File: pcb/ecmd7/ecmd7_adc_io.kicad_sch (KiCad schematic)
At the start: 72 parts, among them U10 FIN1002M5X, U11 FIN1002M5X, U12 FIN1002M5X, U13 ADM3490ExR, U2 MCP33151-05T-E/MN, U4 MCP33151-05T-E/MN, U5 MCP33151-05T-E/MN, U7 MCP33151-05T-E/MN

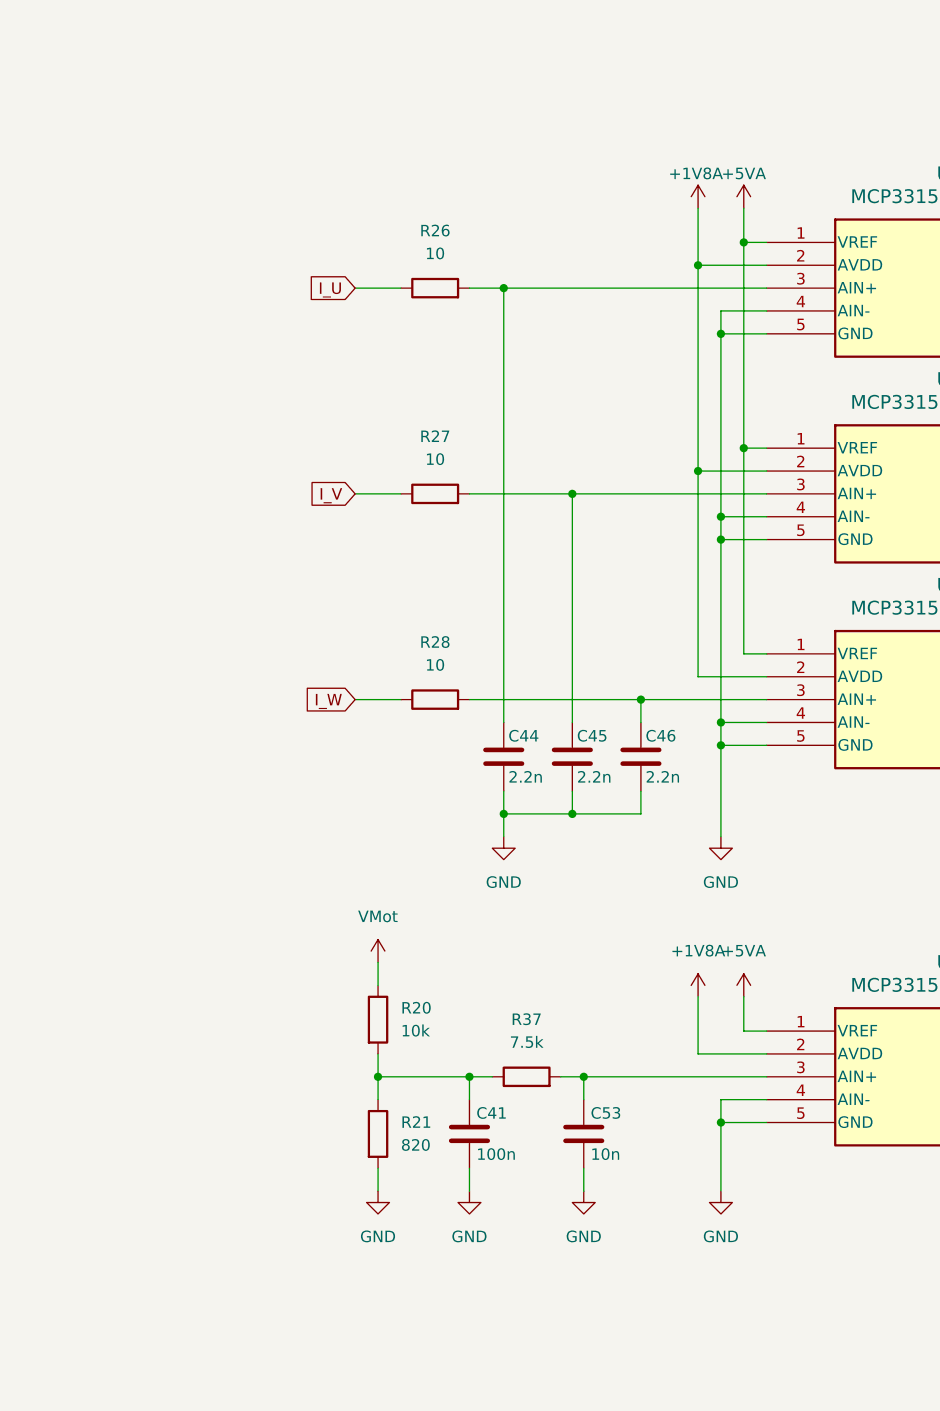
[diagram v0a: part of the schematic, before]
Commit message: WIP: Power stage and ADC routing
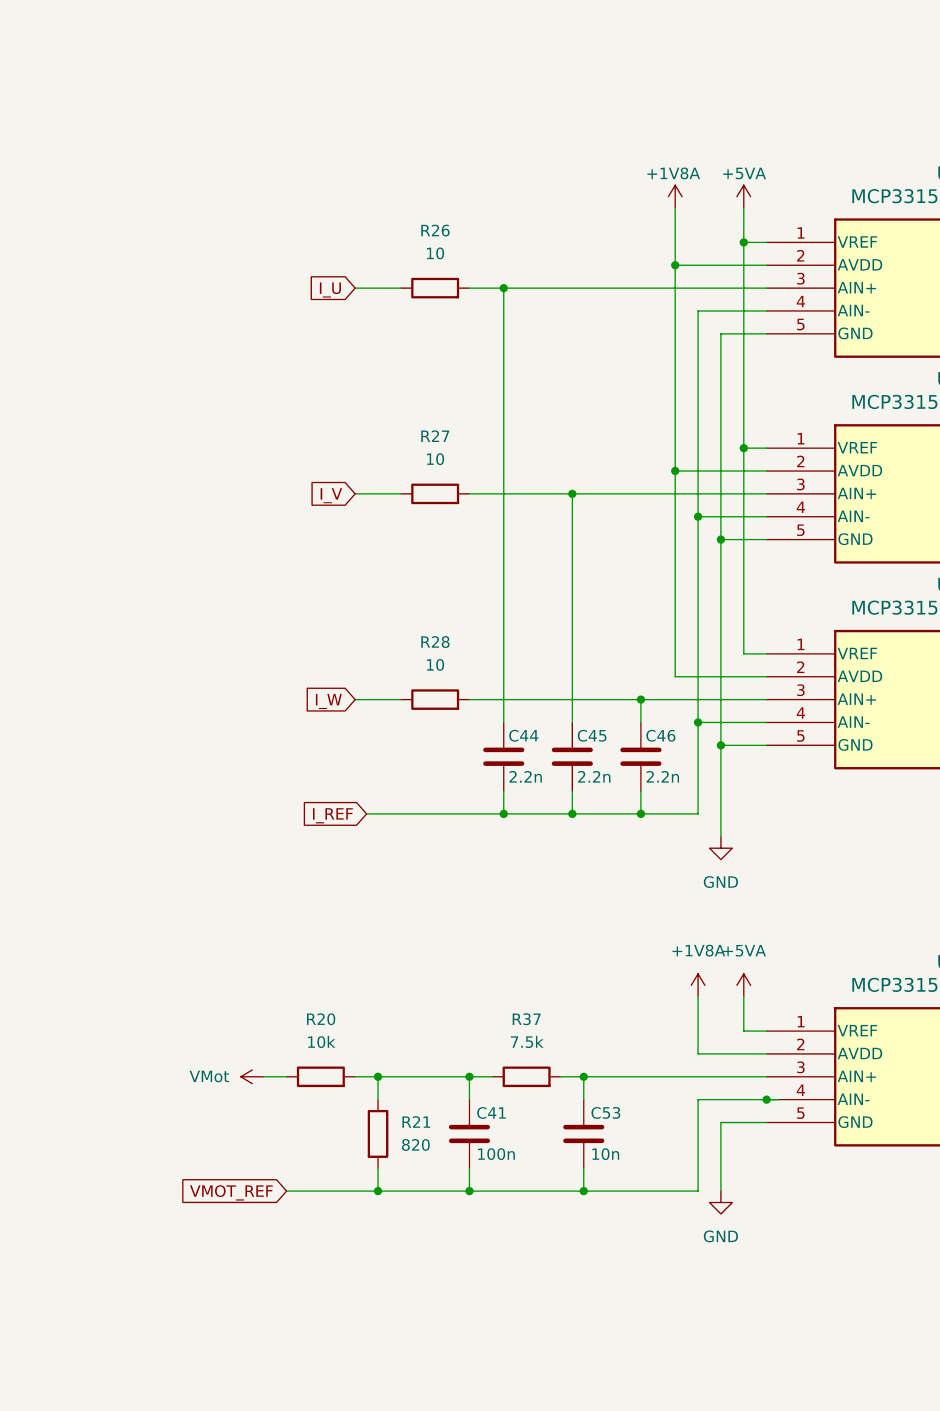
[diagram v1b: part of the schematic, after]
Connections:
- net GND: no longer C41.2, C44.2, C45.2, C46.2, C53.2, R21.2, U2.4 (AIN-), U4.4 (AIN-), U5.4 (AIN-), U7.4 (AIN-)
- new net I_REF: C44.2, C45.2, C46.2, U2.4 (AIN-), U4.4 (AIN-), U5.4 (AIN-)
- new net VMOT_REF: C41.2, C53.2, R21.2, U7.4 (AIN-)
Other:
- moved on the sheet: R20
